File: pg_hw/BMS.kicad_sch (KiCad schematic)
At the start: 2 parts, among them U4 TP4056, U5 MAX17048X+T10

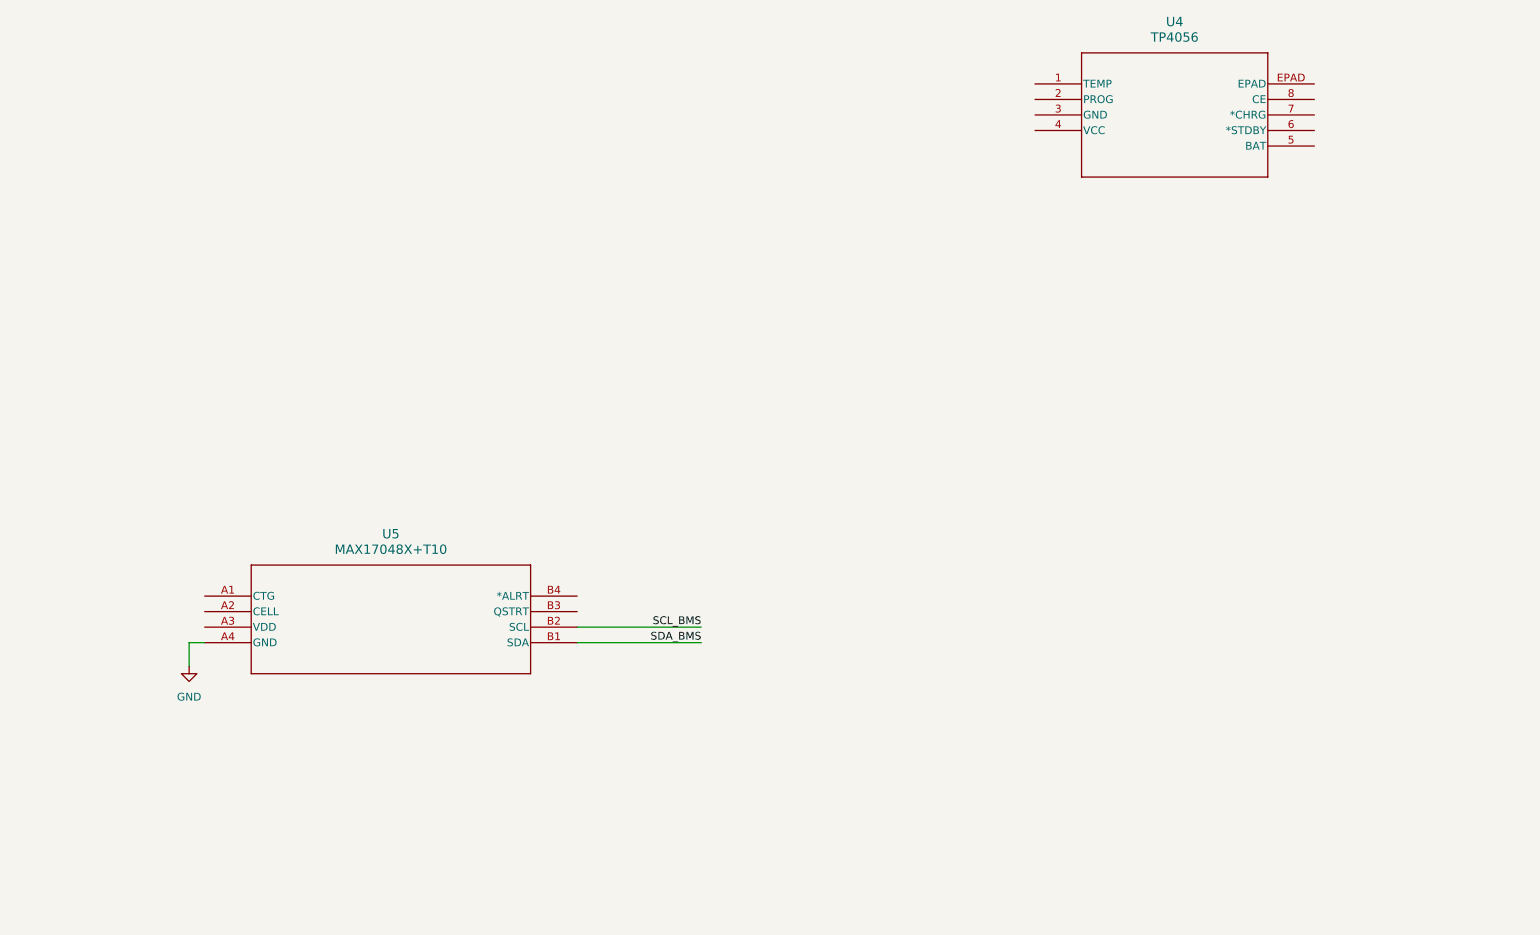
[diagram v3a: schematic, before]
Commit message: change batt again
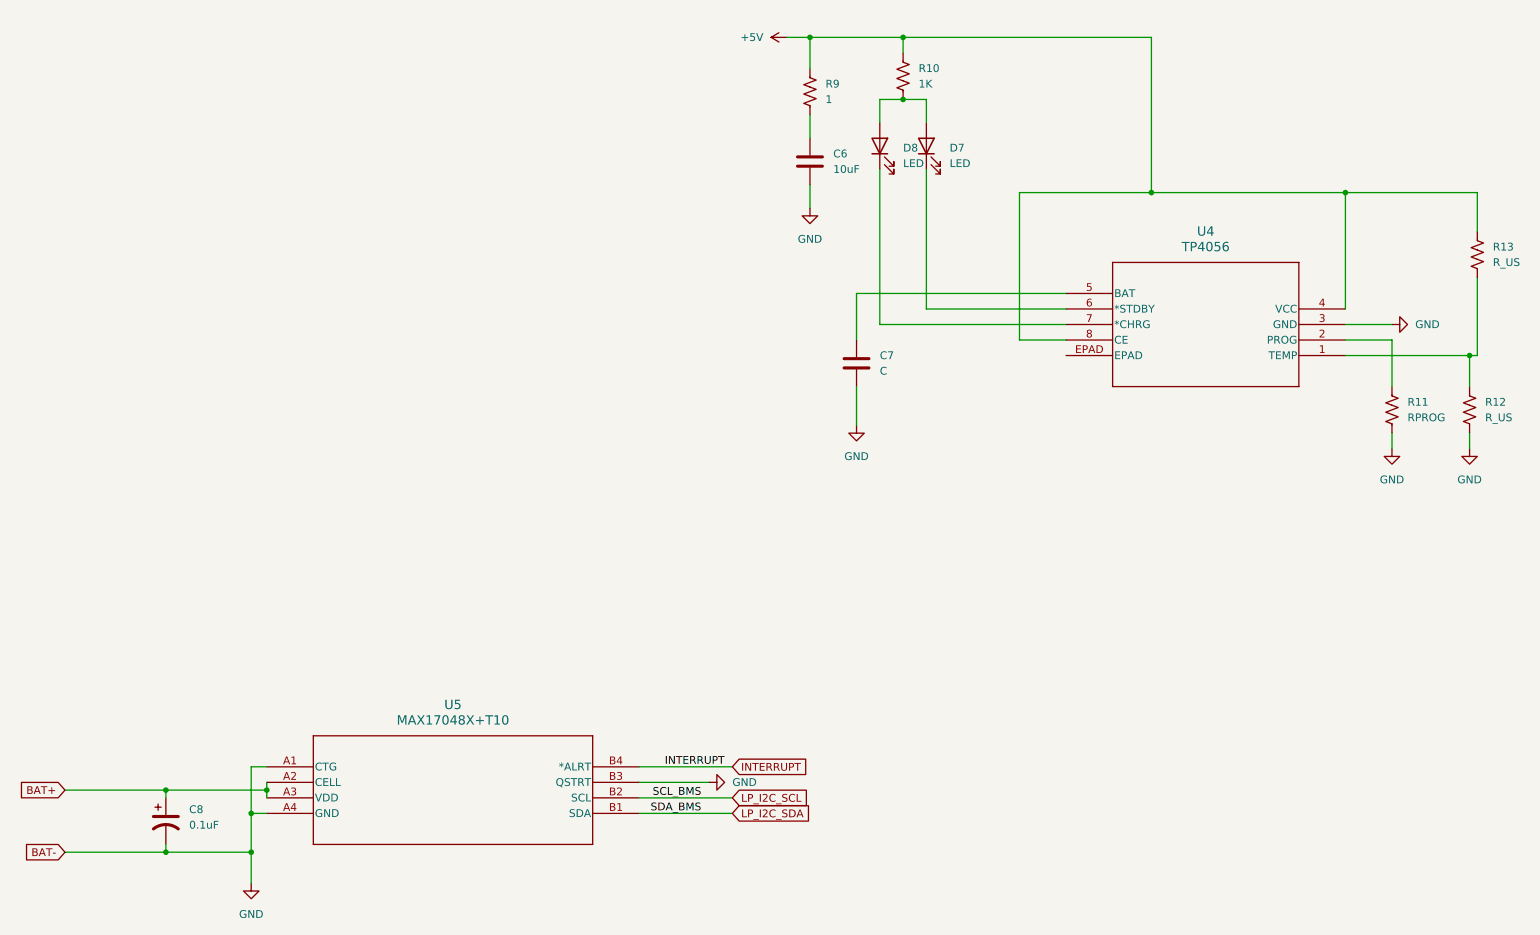
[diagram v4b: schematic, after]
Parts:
- added C6: 10uF, symbol Device:C
- added C7: C, symbol Device:C
- added C8: 0.1uF, symbol Device:C_Polarized_US
- added D7, D8: LED, symbol Device:LED
- added R10: 1K, symbol Device:R_US
- added R11: RPROG, symbol Device:R_US
- added R12, R13: R_US, symbol Device:R_US
- added R9: 1, symbol Device:R_US
- U4: footprint SOP8-PP_TPW -> Package_SO:MSOP-8-1EP_3x3mm_P0.65mm_EP1.5x1.8mm
- U5: footprint 21-0555B_W80B1-1_MXM -> Package_SO:MSOP-8-1EP_3x3mm_P0.65mm_EP1.73x1.85mm
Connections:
- net GND: now also U4.3 (GND), U5.A1 (CTG), U5.B3 (QSTRT), C6.2, C7.2, C8.2, R11.2, R12.2
- net at U4.1 (TEMP): now also R12.1, R13.2
- net at U4.2 (PROG): now also R11.1
- net +5V: now reaches U4.4 (VCC)
- net +5V: now also U4.8 (CE), R10.1, R13.1, R9.1
- net at U4.5 (BAT): now also C7.1
- net at U4.6 (*STDBY): now also D7.1 (K)
- net at U4.7 (*CHRG): now also D8.1 (K)
- net BAT+: now reaches U5.A2 (CELL)
- net BAT+: now also U5.A3 (VDD), C8.1
- net INTERRUPT: now reaches U5.B4 (*ALRT)
- net SCL_BMS renamed LP_I2C_SCL
- net SDA_BMS renamed LP_I2C_SDA
- new net: C6.1, R9.2
- new net: D7.2 (A), D8.2 (A), R10.2
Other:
- moved on the sheet: U4, U5

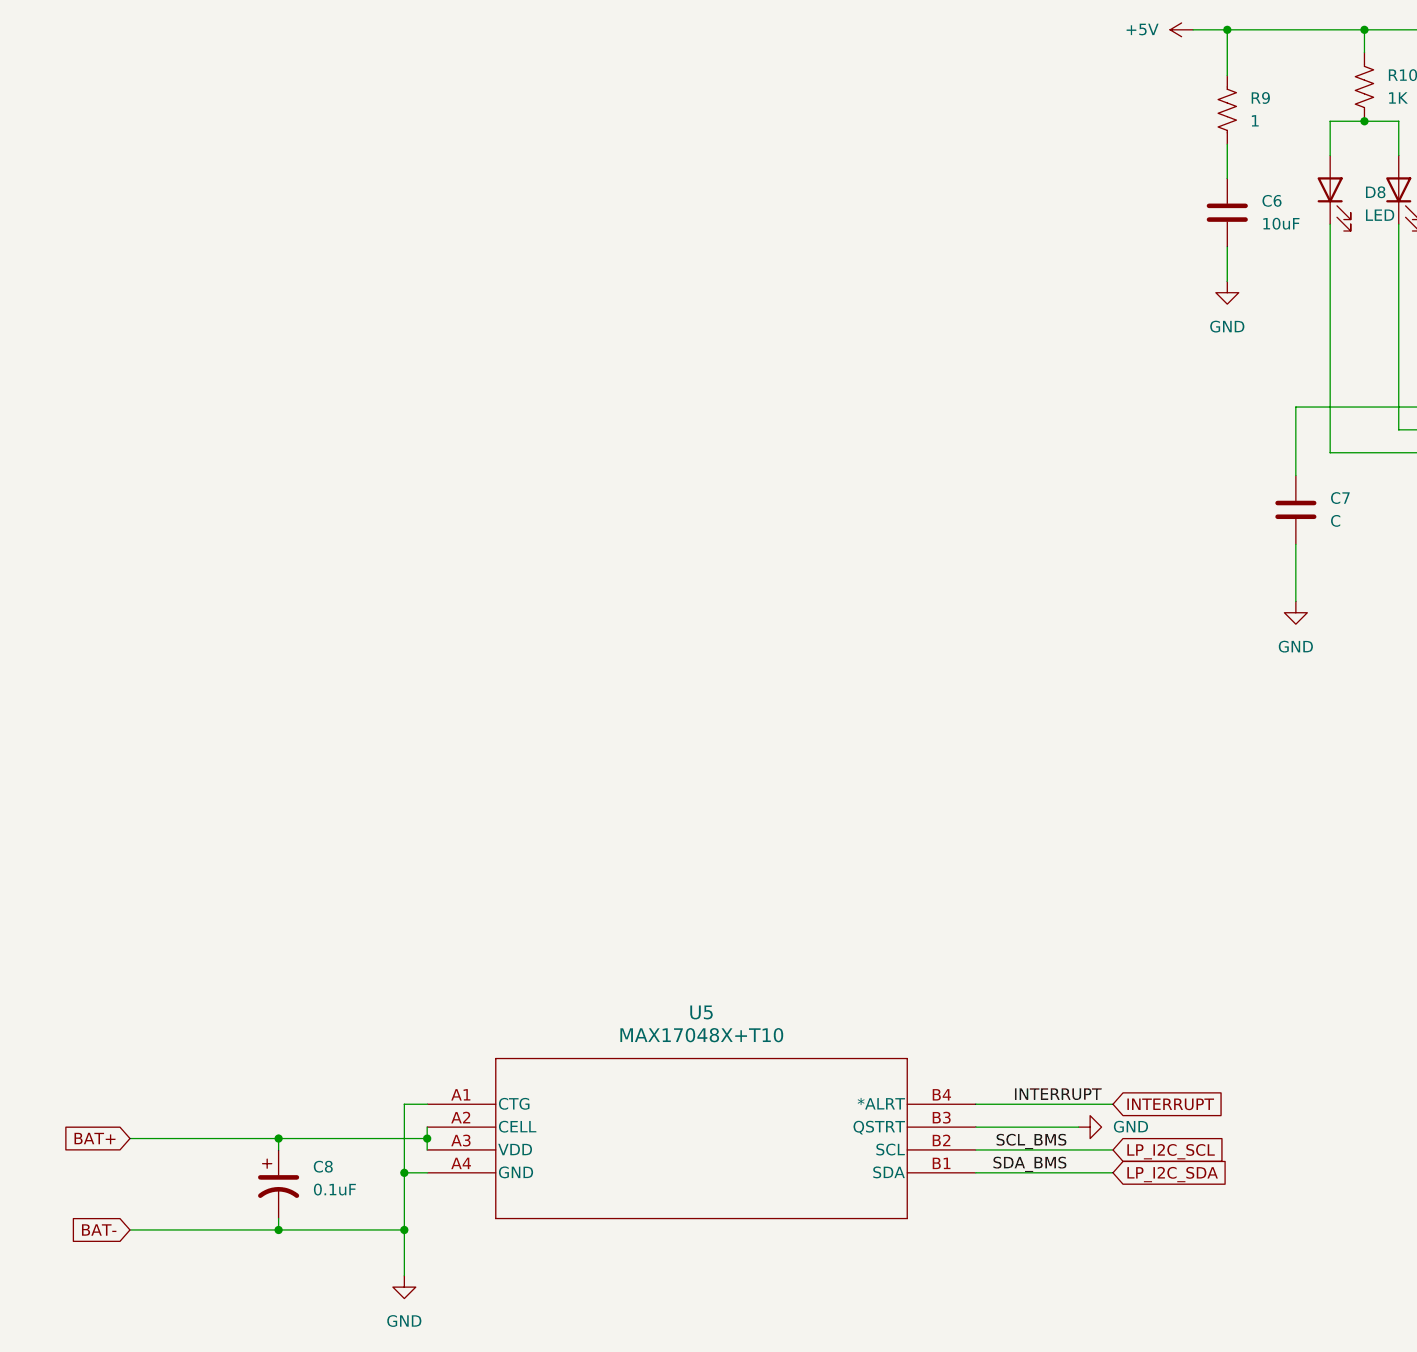
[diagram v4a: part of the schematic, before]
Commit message: hui
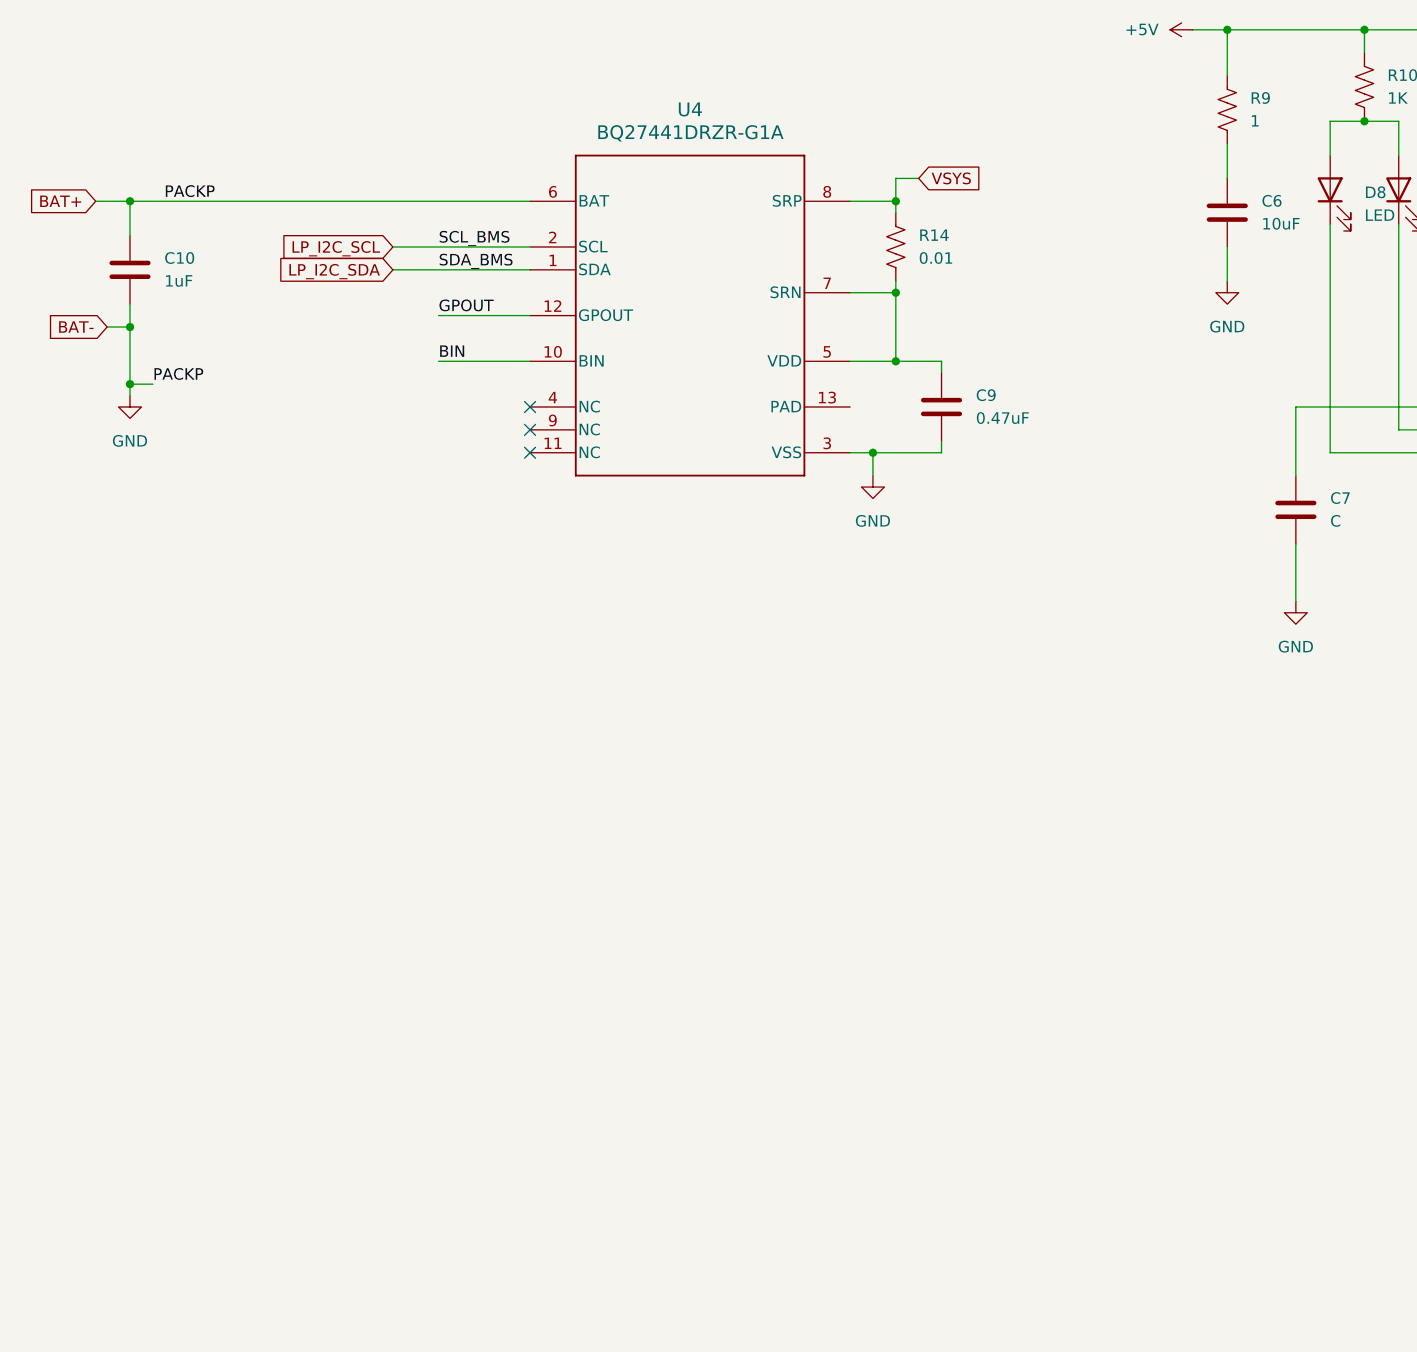
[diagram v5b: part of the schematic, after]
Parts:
- removed C8: 0.1uF, symbol Device:C_Polarized_US
- removed U5: MAX17048X+T10, Package_SO:MSOP-8-1EP_3x3mm_P0.65mm_EP1.73x1.85mm, symbol ul_MAX17048X-T10:MAX17048X+T10
- added C10: 1uF, Capacitor_SMD:C_0603_1608Metric, symbol Device:C
- added C9: 0.47uF, Resistor_SMD:R_0603_1608Metric, symbol Device:C
- added R14: 0.01, Resistor_SMD:R_0402_1005Metric, symbol Device:R_US
- added U4: BQ27441DRZR-G1A, Copy of DRZ0012A, symbol BQ27441DRZR_G1A:BQ27441DRZR-G1A
- R10, R11, R12, R13, R9: footprint (none) -> Resistor_SMD:R_0402_1005Metric
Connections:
- net GND: now also C10.1, C10.2, C9.2, U4.3 (VSS), U4.6 (BAT)
- net LP_I2C_SCL: now also U4.2 (SCL)
- net LP_I2C_SDA: now also U4.1 (SDA)
- new net: C9.1, R14.2, U4.5 (VDD), U4.7 (SRN)
- new net BIN: U4.10 (BIN)
- new net GPOUT: U4.12 (GPOUT)
- new net VSYS: R14.1, U4.8 (SRP)
- no-connect marks 0 -> 3
